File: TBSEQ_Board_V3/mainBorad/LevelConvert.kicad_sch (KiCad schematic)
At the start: 8 parts, among them J10 Conn_01x05, J11 Conn_01x05, J4 Conn_01x03, J5 Conn_01x03

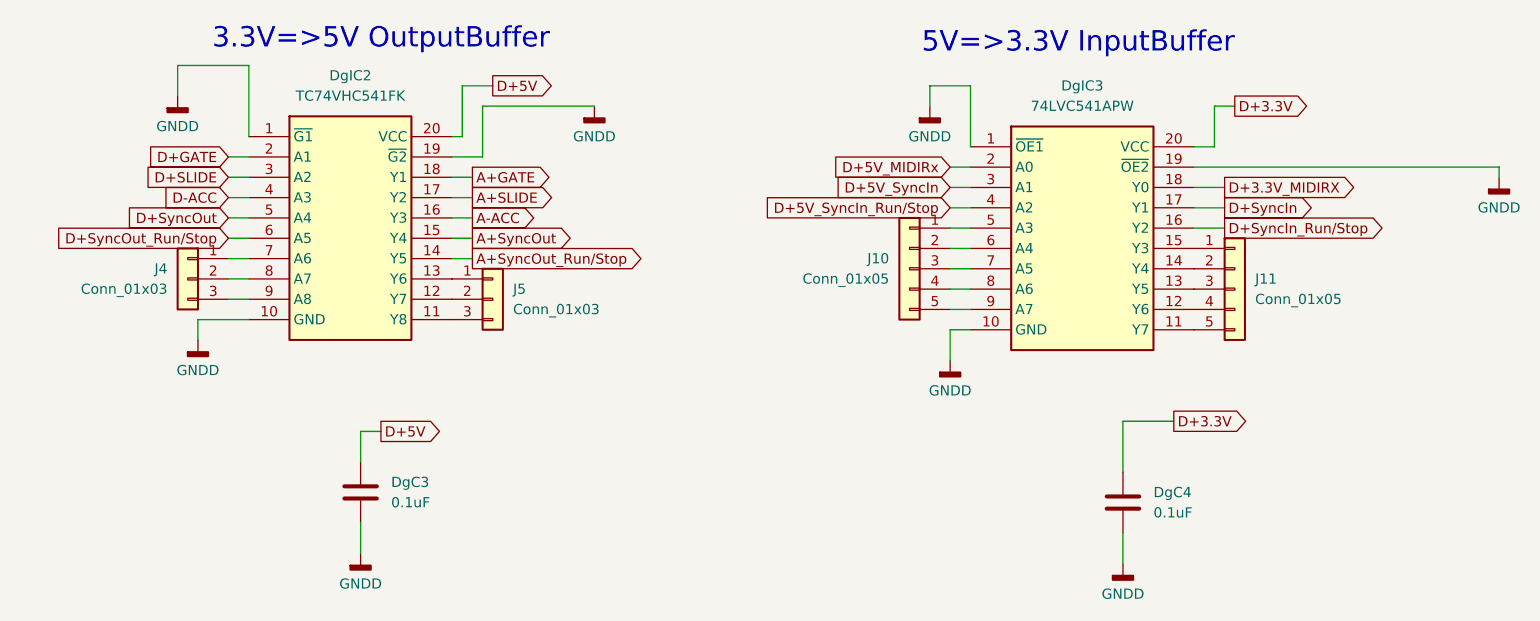
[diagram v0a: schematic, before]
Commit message: V3Board
アートワーク中
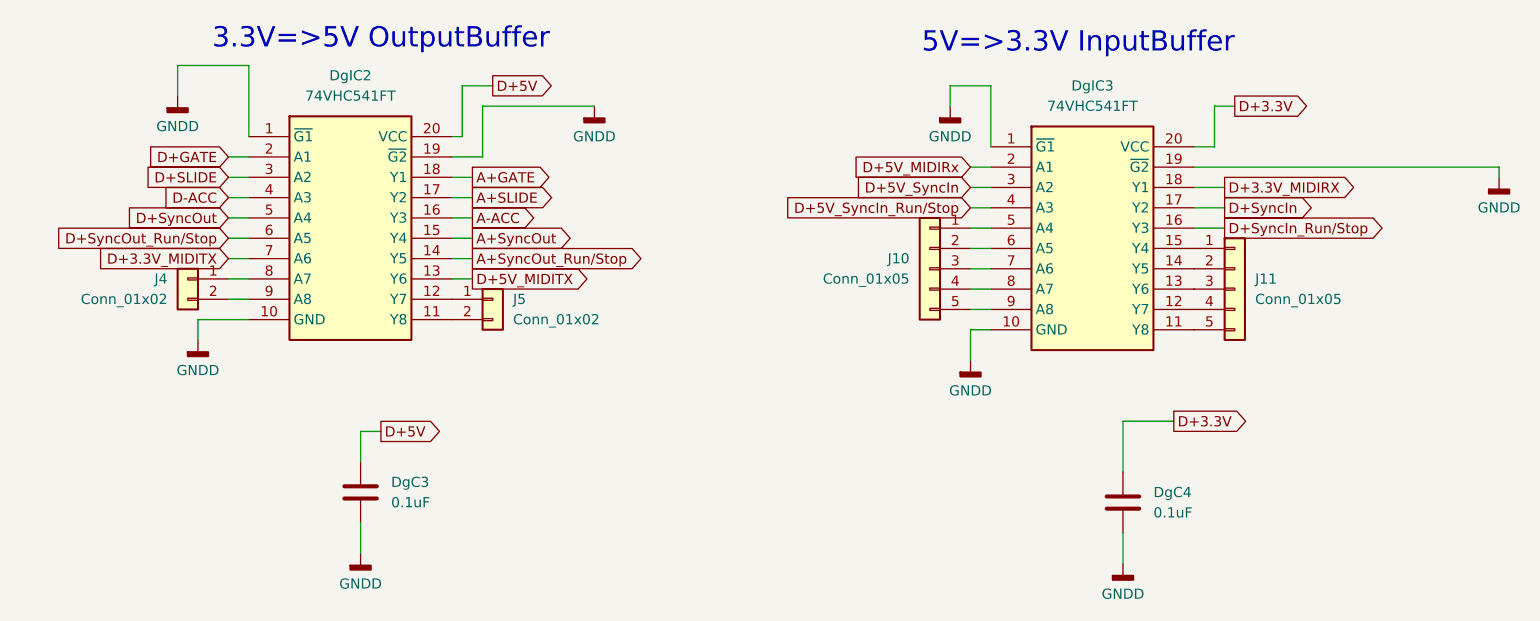
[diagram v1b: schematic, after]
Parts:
- removed DgIC2: TC74VHC541FK, SamacSys_Parts:SOP50P400X100-20N, symbol SamacSys_Parts:TC74VHC541FK
- removed DgIC3: 74LVC541APW, SOP65P640X110-20N, symbol SamacSys_Parts:74LVC541APW
- removed J4, J5: Conn_01x03, Connector_PinHeader_2.54mm:PinHeader_1x03_P2.54mm_Vertical, symbol Connector_Generic:Conn_01x03
- added DgIC2, DgIC3: 74VHC541FT, SamacSys_Parts:SOP65P640X120-20N, symbol SamacSys_Parts:74VHC541FT
- added J4, J5: Conn_01x02, Connector_PinHeader_2.54mm:PinHeader_1x02_P2.54mm_Vertical, symbol Connector_Generic:Conn_01x02
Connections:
- net A+GATE: now also DgIC2.18 (Y1)
- net A+SLIDE: now also DgIC2.17 (Y2)
- net A+SyncOut: now also DgIC2.15 (Y4)
- net A+SyncOut_Run/Stop: now also DgIC2.14 (Y5)
- net A-ACC: now also DgIC2.16 (Y3)
- net D+3.3V: now also DgIC3.20 (VCC)
- net D+3.3V_MIDIRX: now also DgIC3.18 (Y1)
- net D+5V: now also DgIC2.20 (VCC)
- net D+5V_MIDIRx: now also DgIC3.2 (A1)
- net D+5V_SyncIn: now also DgIC3.3 (A2)
- net D+5V_SyncIn_Run/Stop: now also DgIC3.4 (A3)
- net D+GATE: now also DgIC2.2 (A1)
- net D+SLIDE: now also DgIC2.3 (A2)
- net D+SyncIn: now also DgIC3.17 (Y2)
- net D+SyncIn_Run/Stop: now also DgIC3.16 (Y3)
- net D+SyncOut: now also DgIC2.5 (A4)
- net D+SyncOut_Run/Stop: now also DgIC2.6 (A5)
- net D-ACC: now also DgIC2.4 (A3)
- net GNDD: now also DgIC2.1 (~{G1}), DgIC2.10 (GND), DgIC2.19 (~{G2}), DgIC3.1 (~{G1}), DgIC3.10 (GND), DgIC3.19 (~{G2})
- net at J11.5 (Pin_5): now also DgIC3.11 (Y8)
- net at J11.4 (Pin_4): now also DgIC3.12 (Y7)
- net at J11.3 (Pin_3): now also DgIC3.13 (Y6)
- net at J11.2 (Pin_2): now also DgIC3.14 (Y5)
- net at J11.1 (Pin_1): now also DgIC3.15 (Y4)
- net at J10.1 (Pin_1): now also DgIC3.5 (A4)
- net at J10.2 (Pin_2): now also DgIC3.6 (A5)
- net at J10.3 (Pin_3): now also DgIC3.7 (A6)
- net at J10.4 (Pin_4): now also DgIC3.8 (A7)
- net at J10.5 (Pin_5): now also DgIC3.9 (A8)
- new net: DgIC2.12 (Y7), J5.1 (Pin_1)
- new net: DgIC2.11 (Y8), J5.2 (Pin_2)
- new net: DgIC2.8 (A7), J4.1 (Pin_1)
- new net: DgIC2.9 (A8), J4.2 (Pin_2)
- new net D+3.3V_MIDITX: DgIC2.7 (A6)
- new net D+5V_MIDITX: DgIC2.13 (Y6)
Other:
- moved on the sheet: J10
